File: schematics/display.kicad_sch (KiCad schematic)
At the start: 62 parts, among them Q10 S8550, Q11 S8550, Q12 TN2106, Q13 TN2106, Q14 TN2106, Q15 TN2106, Q16 TN2106, Q17 TN2106, Q18 TN2106, Q2 TN2106, Q3 TN2106, Q4 S8550, Q5 S8550, Q6 S8550, Q7 S8550, Q8 S8550, Q9 S8550, U16 5161BS, U17 74HC251, U18 74HC251, U19 74HC251, U20 74HC251, U21 74HC138, U22 74HC4511, U23 5161BS, U24 5161BS, U25 5161BS, U26 5161BS, U27 5161BS, U28 5161BS, U29 5161BS, U30 5161BS

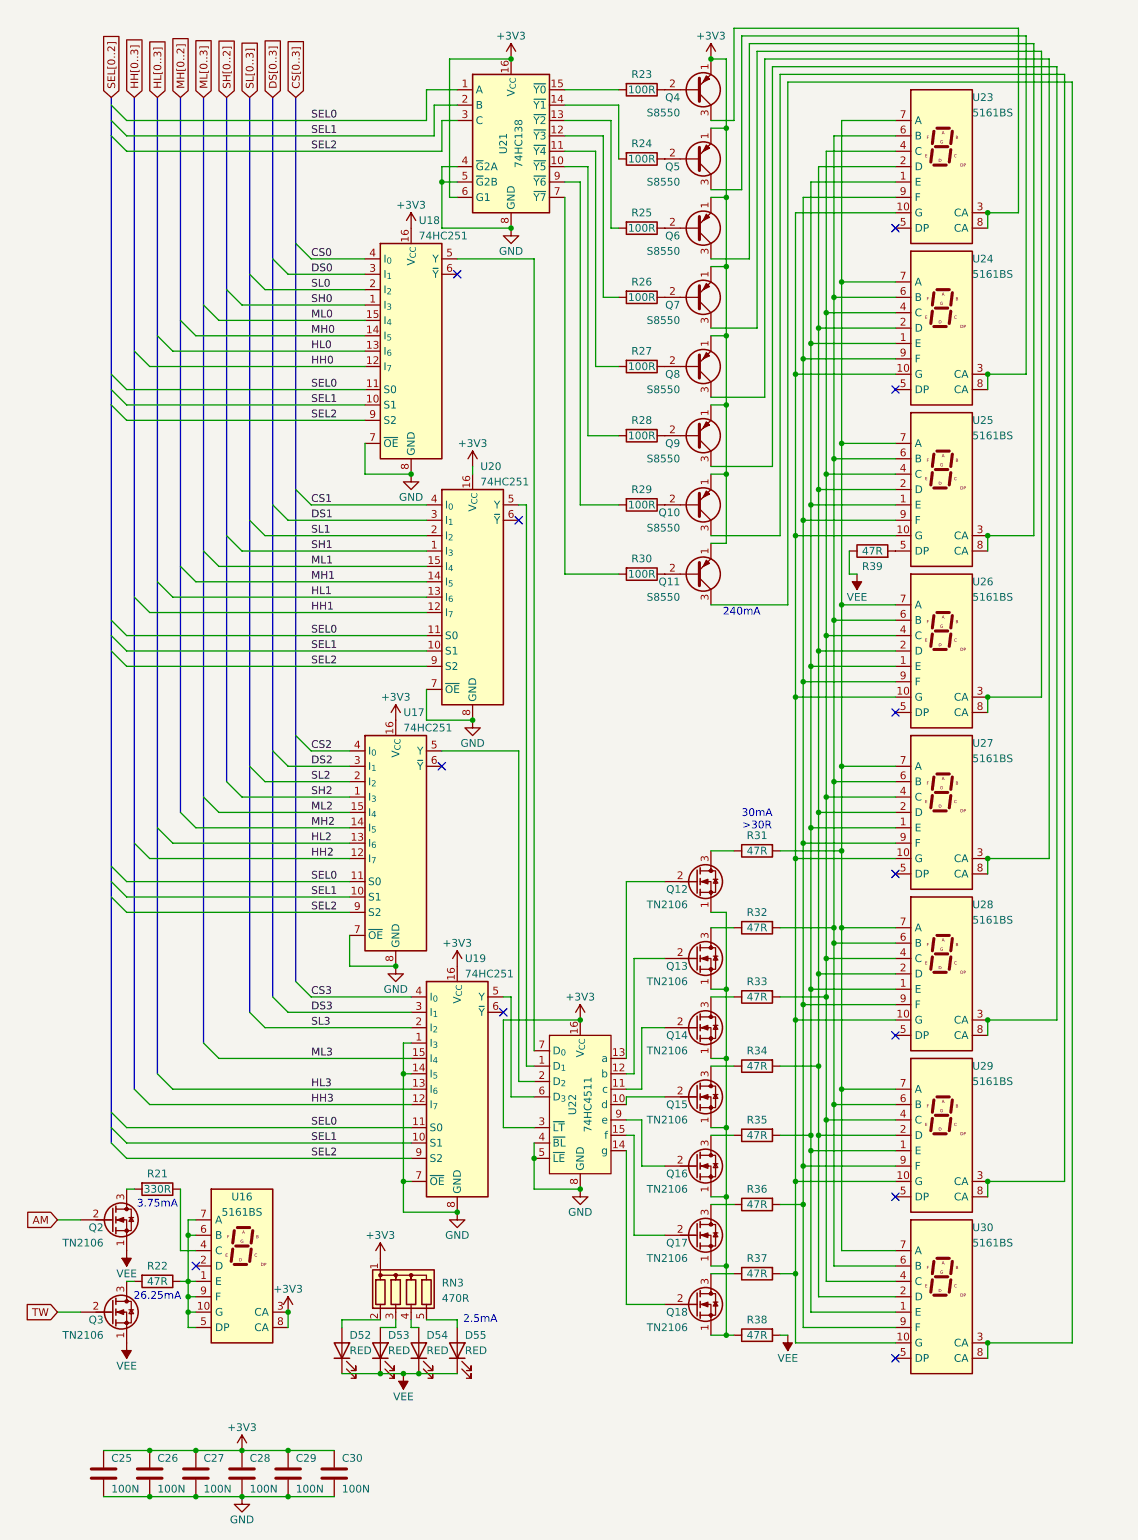
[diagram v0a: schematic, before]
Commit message: preliminary PCB design
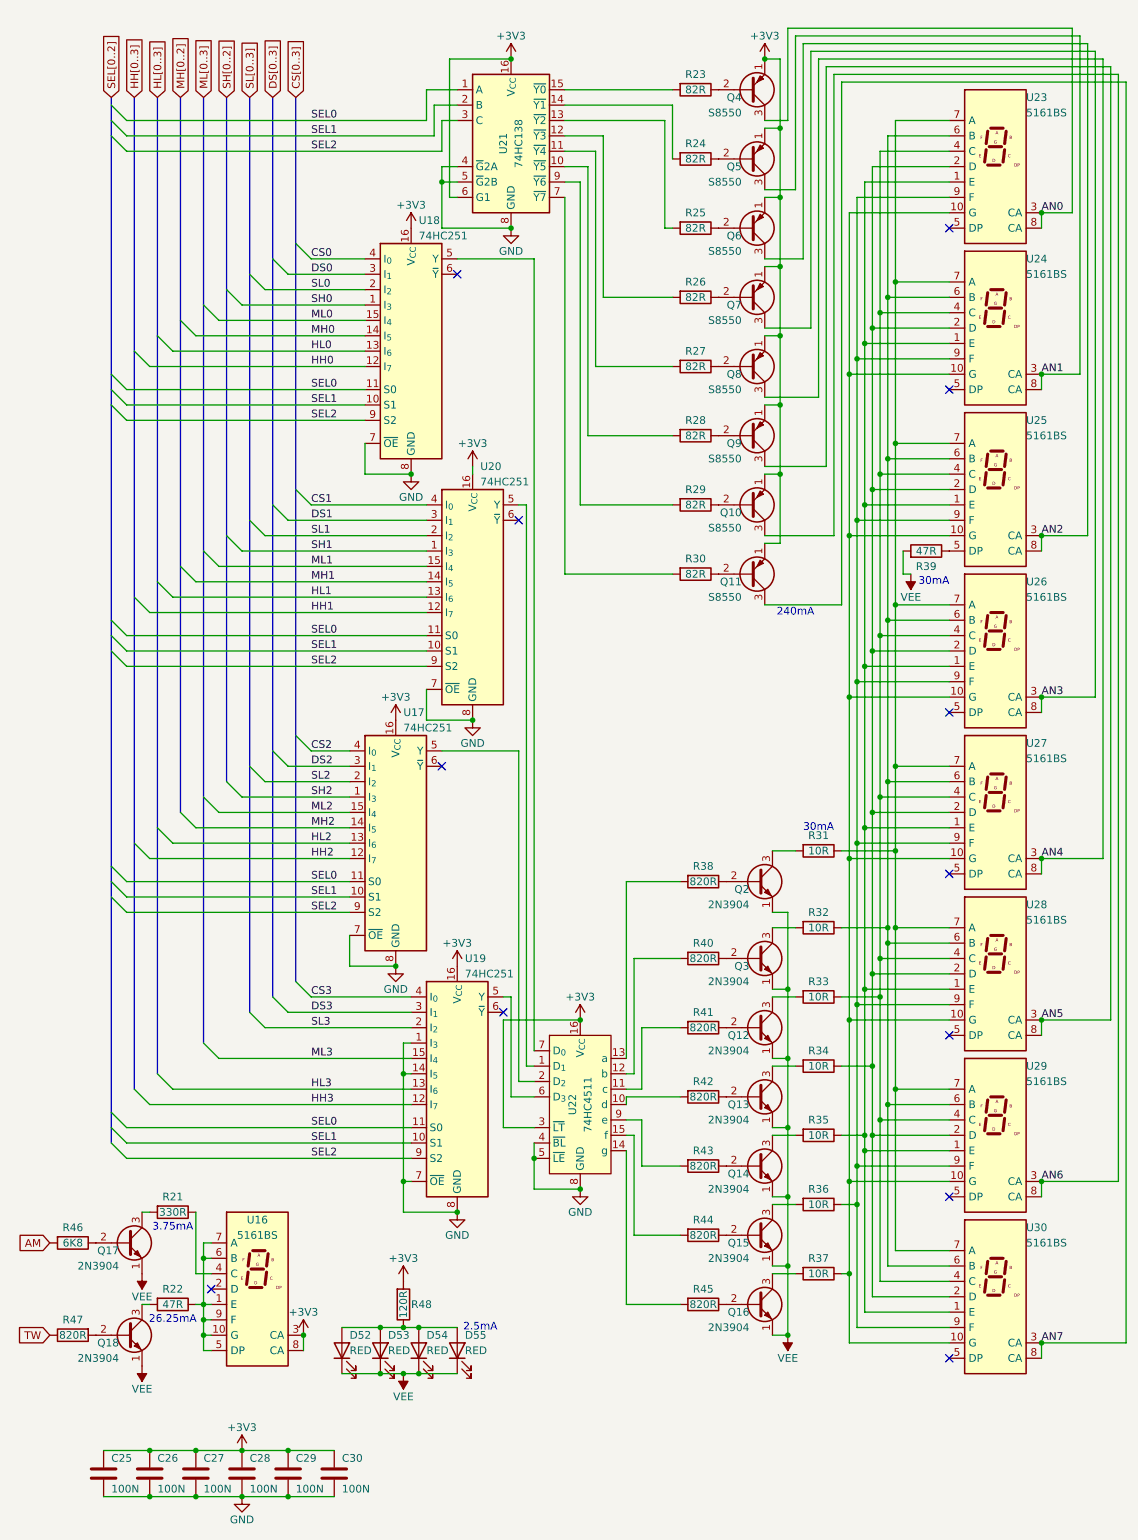
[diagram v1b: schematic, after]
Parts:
- removed Q12, Q13, Q14, Q15, Q16, Q17, Q18, Q2, Q3: TN2106, Package_TO_SOT_THT:TO-92_HandSolder, symbol Transistor_FET:Q_NMOS_SGD
- removed RN3: 470R, Resistor_THT:R_Array_SIP5, symbol Device:R_Network04
- added Q12, Q13, Q14, Q15, Q16, Q17, Q18, Q2, Q3: 2N3904, Package_TO_SOT_THT:TO-92_HandSolder, symbol Transistor_BJT:2N3904
- added R40, R41, R42, R43, R44, R45, R47: 820R, bvclock:THT_R_Vertical, symbol Device:R
- added R46: 6K8, bvclock:THT_R_Vertical, symbol Device:R
- added R48: 120R, bvclock:THT_R_Vertical, symbol Device:R
- C25, C26, C27, C28, C29, C30: footprint Capacitor_THT:C_Disc_D5.1mm_W3.2mm_P5.00mm -> bvclock:THT_Cap
- R21, R22, R39: footprint Resistor_THT:R_Axial_DIN0207_L6.3mm_D2.5mm_P7.62mm_Horizontal -> bvclock:THT_R_Vertical
- R23, R24, R25, R26, R27, R28, R29, R30: value 100R -> 82R; footprint Resistor_THT:R_Axial_DIN0207_L6.3mm_D2.5mm_P7.62mm_Horizontal -> bvclock:THT_R_Vertical
- R31, R32, R33, R34, R35, R36, R37: value 47R -> 10R; footprint Resistor_THT:R_Axial_DIN0207_L6.3mm_D2.5mm_P7.62mm_Horizontal -> bvclock:THT_R_Vertical
- R38: value 47R -> 820R; footprint Resistor_THT:R_Axial_DIN0207_L6.3mm_D2.5mm_P7.62mm_Horizontal -> bvclock:THT_R_Vertical
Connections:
- net +3V3: now also R48.2
- net AM: now also R46.2
- net TW: now also R47.1
- net VEE: now also R39.2, Q12.1 (E), Q13.1 (E), Q14.1 (E), Q15.1 (E), Q16.1 (E), Q17.1 (E), Q18.1 (E), Q2.1 (E), Q3.1 (E); no longer R38.2, R39.1
- net at U23.1 (E), U24.1 (E), U25.1 (E)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: now also R35.1; no longer R35.2
- net at U23.10 (G), U24.10 (G), U25.10 (G)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: now also R37.1; no longer R37.2
- net at U23.2 (D), U24.2 (D), U25.2 (D)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: now also R34.1; no longer R34.2
- net AN2: now reaches Q6.3 (C), U25.3 (CA), U25.8 (CA)
- net at U23.4 (C), U24.4 (C), U25.4 (C)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: now also R33.1; no longer R33.2
- net at U25.5 (DP): now also R39.1; no longer R39.2
- net at U23.6 (B), U24.6 (B), U25.6 (B)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: now also R32.1; no longer R32.2
- net at U23.7 (A), U24.7 (A), U25.7 (A)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: now also R31.1; no longer R31.2
- net at U23.9 (F), U24.9 (F), U25.9 (F)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: now also R36.1; no longer R36.2
- net AN7: now reaches Q11.3 (C), U30.3 (CA), U30.8 (CA)
- net at D54.2 (A): now also D52.2 (A), D53.2 (A), D55.2 (A), R48.1
- net at R22.2: now also Q18.3 (C)
- net AN0: now reaches Q4.3 (C), U23.3 (CA), U23.8 (CA)
- net at R38.1: now also Q2.2 (B)
- net at U22.14 (g): now also R45.2
- net at U22.11 (c): now also R41.2
- net at R21.2: now also Q17.3 (C)
- net AN4: now reaches Q8.3 (C), U27.3 (CA), U27.8 (CA)
- net AN5: now reaches Q9.3 (C), U28.3 (CA), U28.8 (CA)
- net AN6: now reaches Q10.3 (C), U29.3 (CA), U29.8 (CA)
- net at U22.10 (d): now also R42.2
- net AN3: now reaches Q7.3 (C), U26.3 (CA), U26.8 (CA)
- net at U22.9 (e): now also R43.2
- net at U22.12 (b): now also R40.2
- net AN1: now reaches Q5.3 (C), U24.3 (CA), U24.8 (CA)
- net at U22.13 (a): now also R38.2
- net at U22.15 (f): now also R44.2
- new net: Q12.2 (B), R41.1
- new net: Q14.3 (C), R35.2
- new net: Q13.2 (B), R42.1
- new net: Q15.2 (B), R44.1
- new net: Q15.3 (C), R36.2
- new net: Q16.3 (C), R37.2
- new net: Q3.2 (B), R40.1
- new net: Q13.3 (C), R34.2
- new net: Q18.2 (B), R47.2
- new net: Q17.2 (B), R46.1
- new net: Q12.3 (C), R33.2
- new net: Q14.2 (B), R43.1
- new net: Q3.3 (C), R32.2
- new net: Q2.3 (C), R31.2
- new net: Q16.2 (B), R45.1
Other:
- note added: "30mA"
- note removed: "30mA >30R"
- moved on the sheet: Q10, Q11, Q4, Q5, Q6, Q7, Q8, Q9, R21, R22, R23, R24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

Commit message: fixing DRC violations...
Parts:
- Q10, Q11, Q12, Q13, Q14, Q15, Q16, Q17, Q18, Q2, Q3, Q4, Q5, Q6, Q7, Q8, Q9: footprint Package_TO_SOT_THT:TO-92_HandSolder -> bvclock:TO-92_HandSolder
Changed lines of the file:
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@@
 			)
 		)
-		(property "Footprint" "Package_TO_SOT_THT:TO-92_HandSolder"
+		(property "Footprint" "bvclock:TO-92_HandSolder"
 			(at 139.7 105.41 0)
 			(hide yes)
@@
 			)
 		)
-		(property "Footprint" "Package_TO_SOT_THT:TO-92_HandSolder"
+		(property "Footprint" "bvclock:TO-92_HandSolder"
 			(at 139.7 48.26 0)
 			(hide yes)
@@
 			)
 		)
-		(property "Footprint" "Package_TO_SOT_THT:TO-92_HandSolder"
+		(property "Footprint" "bvclock:TO-92_HandSolder"
 			(at 139.7 25.4 0)
 			(hide yes)
@@
 			)
 		)
-		(property "Footprint" "Package_TO_SOT_THT:TO-92_HandSolder"
+		(property "Footprint" "bvclock:TO-92_HandSolder"
 			(at 140.97 213.995 0)
 			(hide yes)
@@
 			)
 		)
-		(property "Footprint" "Package_TO_SOT_THT:TO-92_HandSolder"
+		(property "Footprint" "bvclock:TO-92_HandSolder"
 			(at 139.7 82.55 0)
 			(hide yes)
@@
 			)
 		)
-		(property "Footprint" "Package_TO_SOT_THT:TO-92_HandSolder"
+		(property "Footprint" "bvclock:TO-92_HandSolder"
 			(at 139.7 93.98 0)
 			(hide yes)
@@
 			)
 		)
-		(property "Footprint" "Package_TO_SOT_THT:TO-92_HandSolder"
+		(property "Footprint" "bvclock:TO-92_HandSolder"
 			(at 140.97 191.135 0)
 			(hide yes)
@@
 			)
 		)
-		(property "Footprint" "Package_TO_SOT_THT:TO-92_HandSolder"
+		(property "Footprint" "bvclock:TO-92_HandSolder"
 			(at 139.7 59.69 0)
 			(hide yes)
@@
 			)
 		)
-		(property "Footprint" "Package_TO_SOT_THT:TO-92_HandSolder"
+		(property "Footprint" "bvclock:TO-92_HandSolder"
 			(at 139.7 71.12 0)
 			(hide yes)
@@
 			)
 		)
-		(property "Footprint" "Package_TO_SOT_THT:TO-92_HandSolder"
+		(property "Footprint" "bvclock:TO-92_HandSolder"
 			(at 140.97 155.575 0)
 			(hide yes)
@@
 			)
 		)
-		(property "Footprint" "Package_TO_SOT_THT:TO-92_HandSolder"
+		(property "Footprint" "bvclock:TO-92_HandSolder"
 			(at 140.97 179.705 0)
 			(hide yes)
@@
 			)
 		)
-		(property "Footprint" "Package_TO_SOT_THT:TO-92_HandSolder"
+		(property "Footprint" "bvclock:TO-92_HandSolder"
 			(at 140.97 168.275 0)
 			(hide yes)
@@
 			)
 		)
-		(property "Footprint" "Package_TO_SOT_THT:TO-92_HandSolder"
+		(property "Footprint" "bvclock:TO-92_HandSolder"
 			(at 139.7 36.83 0)
 			(hide yes)
@@
 			)
 		)
-		(property "Footprint" "Package_TO_SOT_THT:TO-92_HandSolder"
+		(property "Footprint" "bvclock:TO-92_HandSolder"
 			(at 140.97 225.425 0)
 			(hide yes)
@@
 			)
 		)
-		(property "Footprint" "Package_TO_SOT_THT:TO-92_HandSolder"
+		(property "Footprint" "bvclock:TO-92_HandSolder"
 			(at 36.83 230.505 0)
 			(hide yes)
@@
 			)
 		)
-		(property "Footprint" "Package_TO_SOT_THT:TO-92_HandSolder"
+		(property "Footprint" "bvclock:TO-92_HandSolder"
 			(at 140.97 202.565 0)
 			(hide yes)
@@
 			)
 		)
-		(property "Footprint" "Package_TO_SOT_THT:TO-92_HandSolder"
+		(property "Footprint" "bvclock:TO-92_HandSolder"
 			(at 36.83 215.265 0)
 			(hide yes)

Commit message: updated DRC for JLCPCB
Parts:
- D52, D53, D54, D55: footprint LED_THT:LED_D5.0mm -> bvclock:LED_D5.0mm
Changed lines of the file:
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@@
 			)
 		)
-		(property "Footprint" "LED_THT:LED_D5.0mm"
+		(property "Footprint" "bvclock:LED_D5.0mm"
 			(at 80.01 231.14 0)
 			(hide yes)
@@
 			)
 		)
-		(property "Footprint" "LED_THT:LED_D5.0mm"
+		(property "Footprint" "bvclock:LED_D5.0mm"
 			(at 67.31 231.14 0)
 			(hide yes)
@@
 			)
 		)
-		(property "Footprint" "LED_THT:LED_D5.0mm"
+		(property "Footprint" "bvclock:LED_D5.0mm"
 			(at 86.36 231.14 0)
 			(hide yes)
@@
 			)
 		)
-		(property "Footprint" "LED_THT:LED_D5.0mm"
+		(property "Footprint" "bvclock:LED_D5.0mm"
 			(at 73.66 231.14 0)
 			(hide yes)
